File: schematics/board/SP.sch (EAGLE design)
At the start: 29 parts

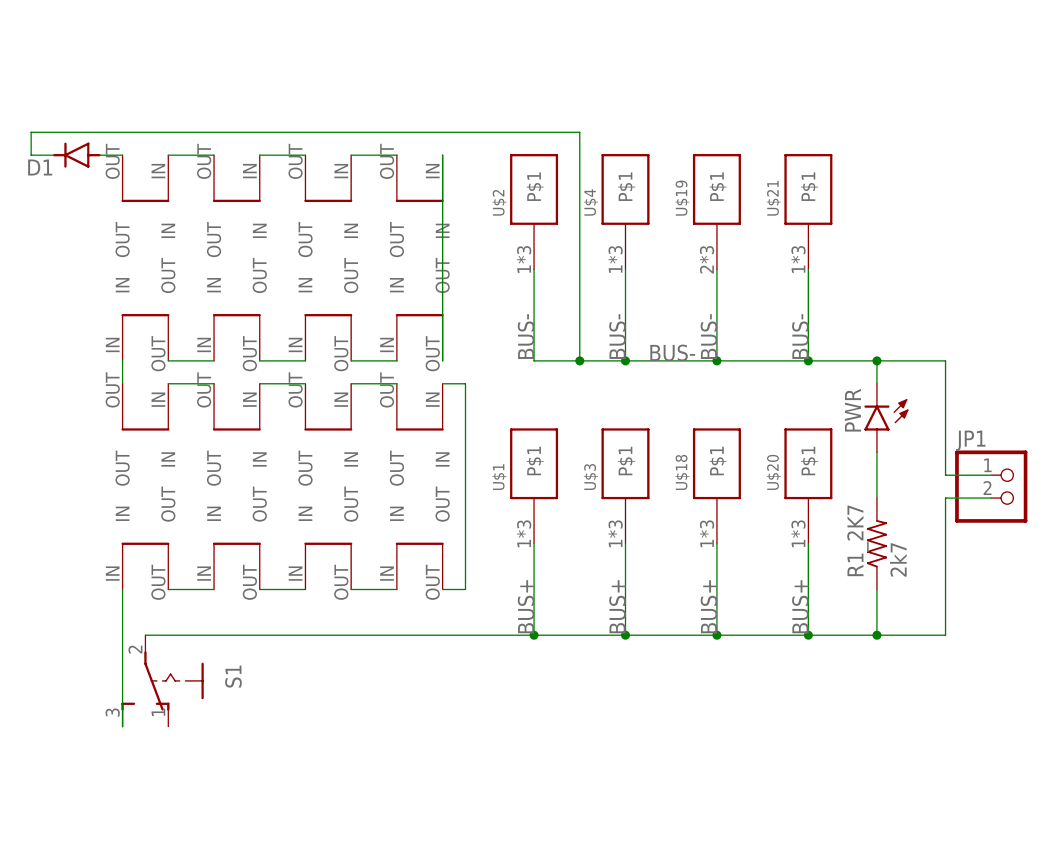
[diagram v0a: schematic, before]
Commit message: Подготовлены к производству платы ARK v1.1 и SP v 1.2
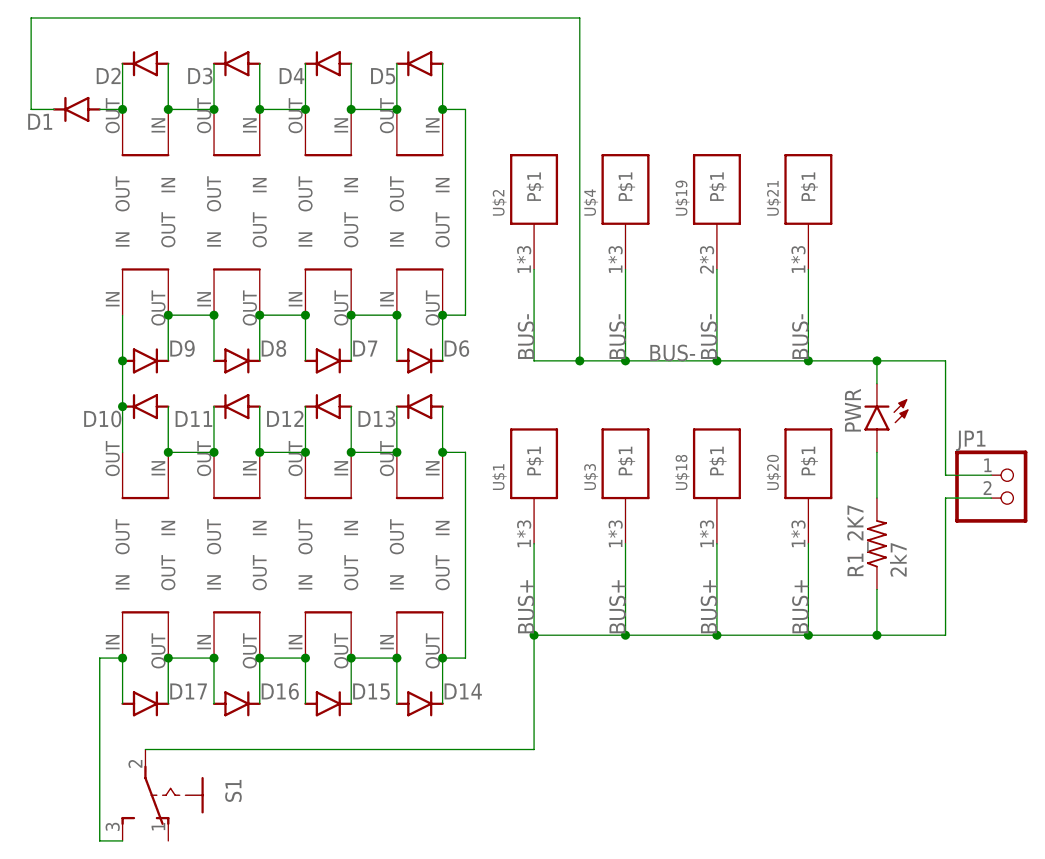
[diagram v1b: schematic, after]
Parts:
- added D10, D11, D12, D13, D14, D15, D16, D17, D2, D3, D4, D5, D6, D7, D8, D9: MBR0520LT, diode:MBR0520LT
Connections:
- net N$1: now also D16.A, D17.C
- net N$10: now also D10.A, D11.C
- net N$11: now also D10.C, D9.A
- net N$12: now also D8.A, D9.C
- net N$13: now also D7.A, D8.C
- net N$14: now also D6.A, D7.C
- net N$15: now also D5.A, D6.C
- net N$16: now also D4.A, D5.C
- net N$17: now also D3.A, D4.C
- net N$18: now also D2.A, D3.C
- net N$24: now also D13.A, D14.C
- net N$3: now also D15.A, D16.C
- net N$4: now also D2.C
- net N$6: now also D14.A, D15.C
- net N$7: now also D17.A
- net N$8: now also D12.A, D13.C
- net N$9: now also D11.A, D12.C
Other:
- moved on the sheet: D1, S1
